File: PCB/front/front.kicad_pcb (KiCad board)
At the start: 2 copper layers, 43 x 26 mm, 22 parts, among them J1 Conn_01x06_Pin, J2 Conn_01x06_Pin, J3 Conn_01x08_Pin, U1 VL53L1CXV0FY1

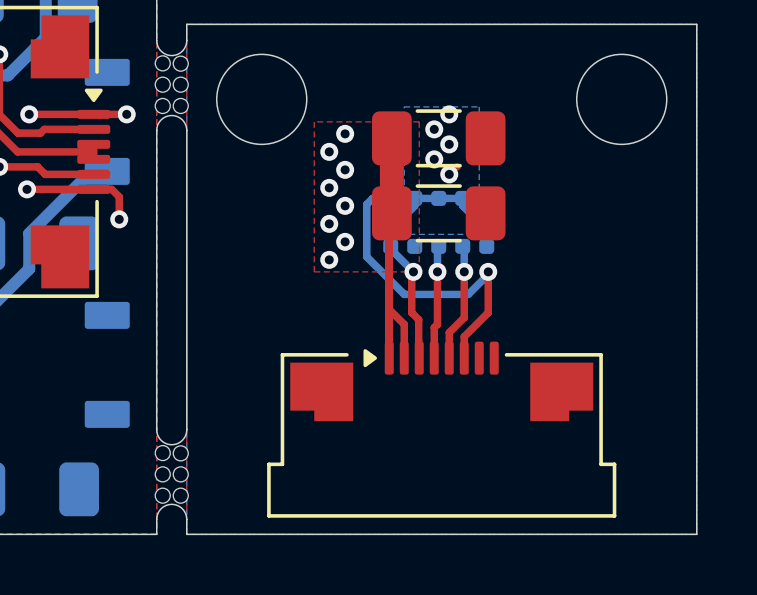
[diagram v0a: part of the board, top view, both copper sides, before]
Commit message: STM32 Mainboard requirements for Programing and Power
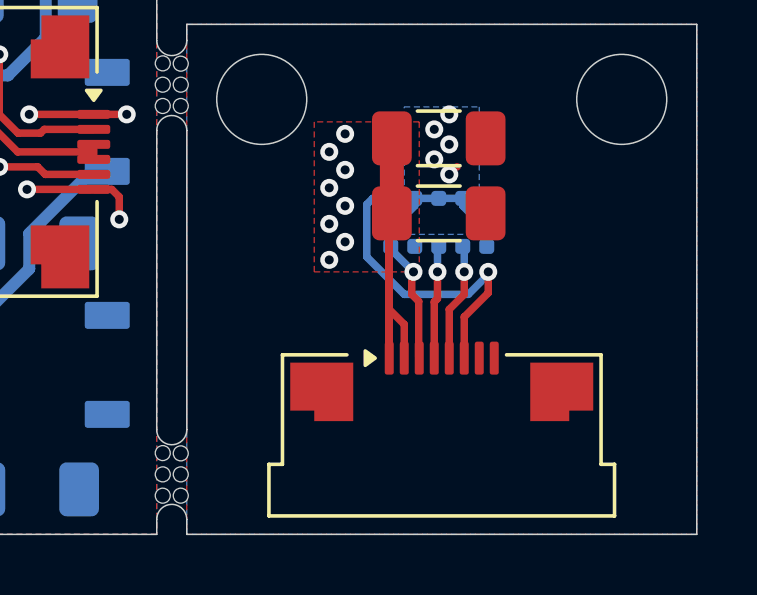
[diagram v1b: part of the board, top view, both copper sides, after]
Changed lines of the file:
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@@
 		)
 		(property "Value" "VL53L1CXV0FY1"
-			(at -0.2 -2.6 -0)
+			(at -0.2 -2.6 0)
 			(layer "F.Fab")
 			(effects
@@
 	)
 	(segment
-		(start 89 129.125)
-		(end 89 128)
+		(start 89 128)
+		(end 88.5 127.5)
 		(width 0.25)
 		(layer "F.Cu")
@@
 	)
 	(segment
-		(start 89 128)
-		(end 88.5 127.5)
-		(width 0.25)
-		(layer "F.Cu")
-		(net 5)
-	)
-	(segment
 		(start 88.5875 121.8)
 		(end 88.5875 124.3)
@@
 	)
 	(segment
+		(start 89 129.125)
+		(end 89 128)
+		(width 0.25)
+		(layer "F.Cu")
+		(net 5)
+	)
+	(segment
 		(start 88.5 128.625)
 		(end 88.5 127.5)
@@
 	)
 	(segment
-		(start 91 126.25)
-		(end 91 127.773108)
+		(start 90.5 127.5)
+		(end 90.5 129.125)
 		(width 0.25)
 		(layer "F.Cu")
@@
 	)
 	(segment
-		(start 91 127.773108)
-		(end 90.5 128.273108)
+		(start 91 126.25)
+		(end 91 127)
 		(width 0.25)
 		(layer "F.Cu")
@@
 	)
 	(segment
-		(start 90.5 128.273108)
-		(end 90.5 129.125)
+		(start 91 127)
+		(end 90.5 127.5)
 		(width 0.25)
 		(layer "F.Cu")
@@
 	)
 	(segment
-		(start 91 129.125)
-		(end 91 128.410918)
+		(start 91 127.75)
+		(end 91.800003 126.949997)
 		(width 0.25)
 		(layer "F.Cu")
@@
 	)
 	(segment
-		(start 91.800003 127.610915)
-		(end 91.800003 126.25)
+		(start 91 129.125)
+		(end 91 127.75)
 		(width 0.25)
 		(layer "F.Cu")
@@
 	)
 	(segment
-		(start 91 128.410918)
-		(end 91.800003 127.610915)
+		(start 91.800003 126.949997)
+		(end 91.800003 126.25)
 		(width 0.25)
 		(layer "F.Cu")
@@
 	)
 	(segment
-		(start 90 128.107772)
-		(end 90 129.125)
+		(start 90.107772 127.142228)
+		(end 90 127.25)
 		(width 0.25)
 		(layer "F.Cu")
@@
 	)
 	(segment
-		(start 90.107772 128)
-		(end 90 128.107772)
+		(start 90 127.25)
+		(end 90 129.125)
 		(width 0.25)
 		(layer "F.Cu")
@@
 	(segment
 		(start 90.107772 126.25)
-		(end 90.107772 128)
+		(end 90.107772 127.142228)
 		(width 0.25)
 		(layer "F.Cu")
@@
 	)
 	(segment
-		(start 89.481772 129.106772)
-		(end 89.5 129.125)
+		(start 89.25 127)
+		(end 89.481772 127.231772)
 		(width 0.25)
 		(layer "F.Cu")
@@
 	(segment
 		(start 89.25 126.307769)
-		(end 89.25 127.61219)
+		(end 89.25 127)
 		(width 0.25)
 		(layer "F.Cu")
@@
 	)
 	(segment
-		(start 89.25 127.61219)
-		(end 89.481772 127.843962)
+		(start 89.481772 129.106772)
+		(end 89.5 129.125)
 		(width 0.25)
 		(layer "F.Cu")
@@
 	)
 	(segment
-		(start 89.481772 127.843962)
+		(start 89.481772 127.231772)
 		(end 89.481772 129.106772)
 		(width 0.25)
